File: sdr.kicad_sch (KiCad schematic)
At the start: 9 parts, among them U1 IS42S86400F-7TL

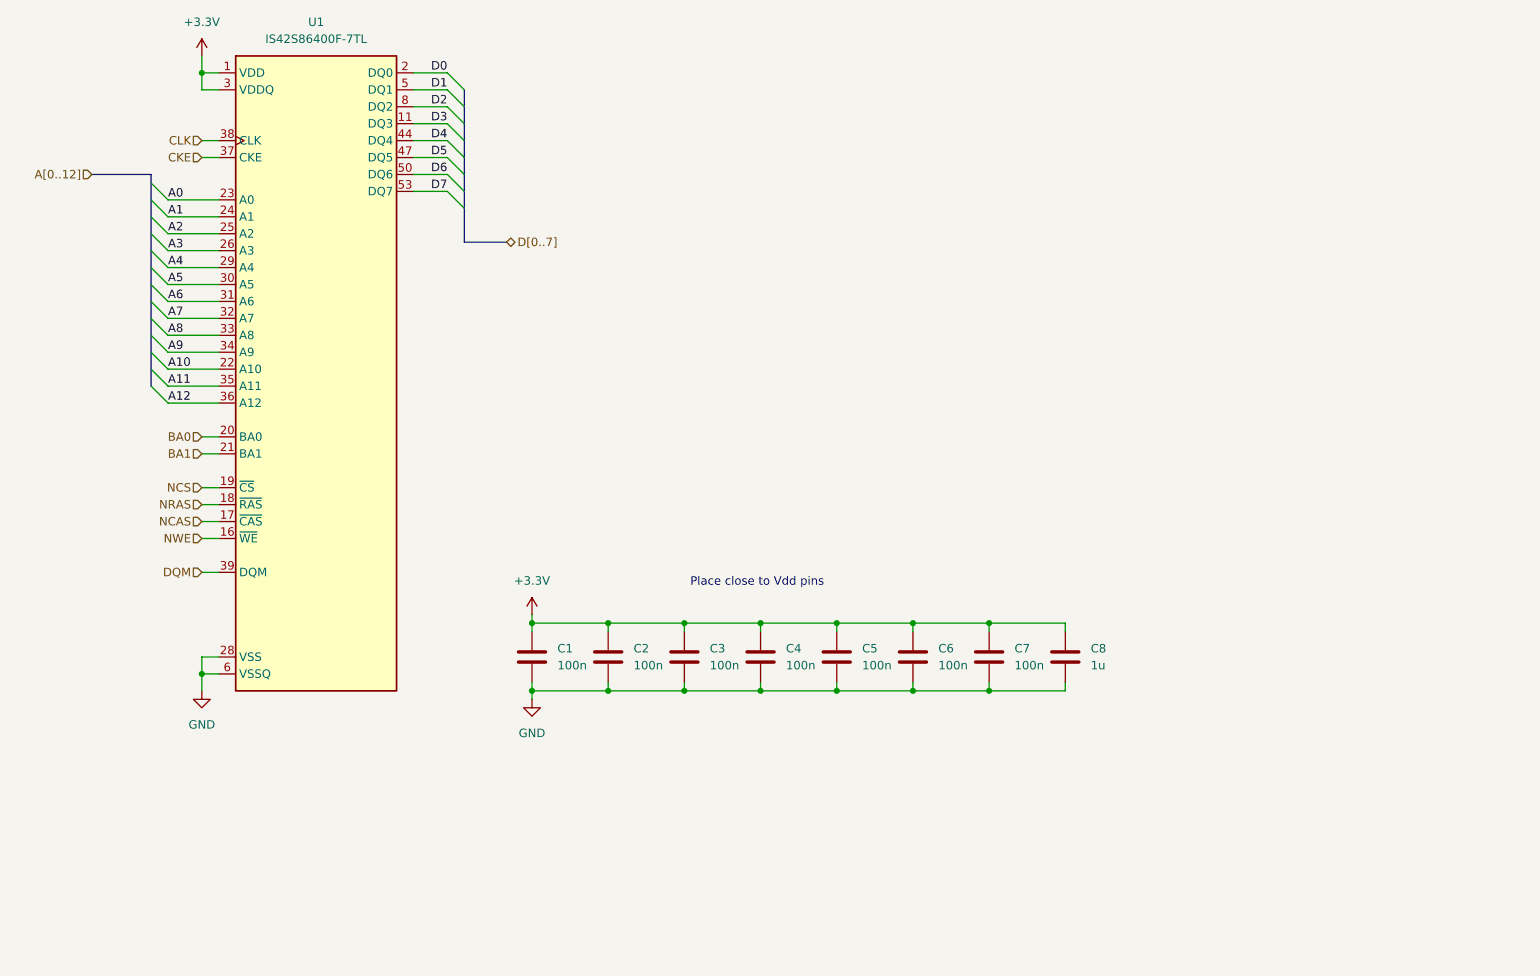
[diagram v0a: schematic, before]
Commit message: [#100650] Add rev number
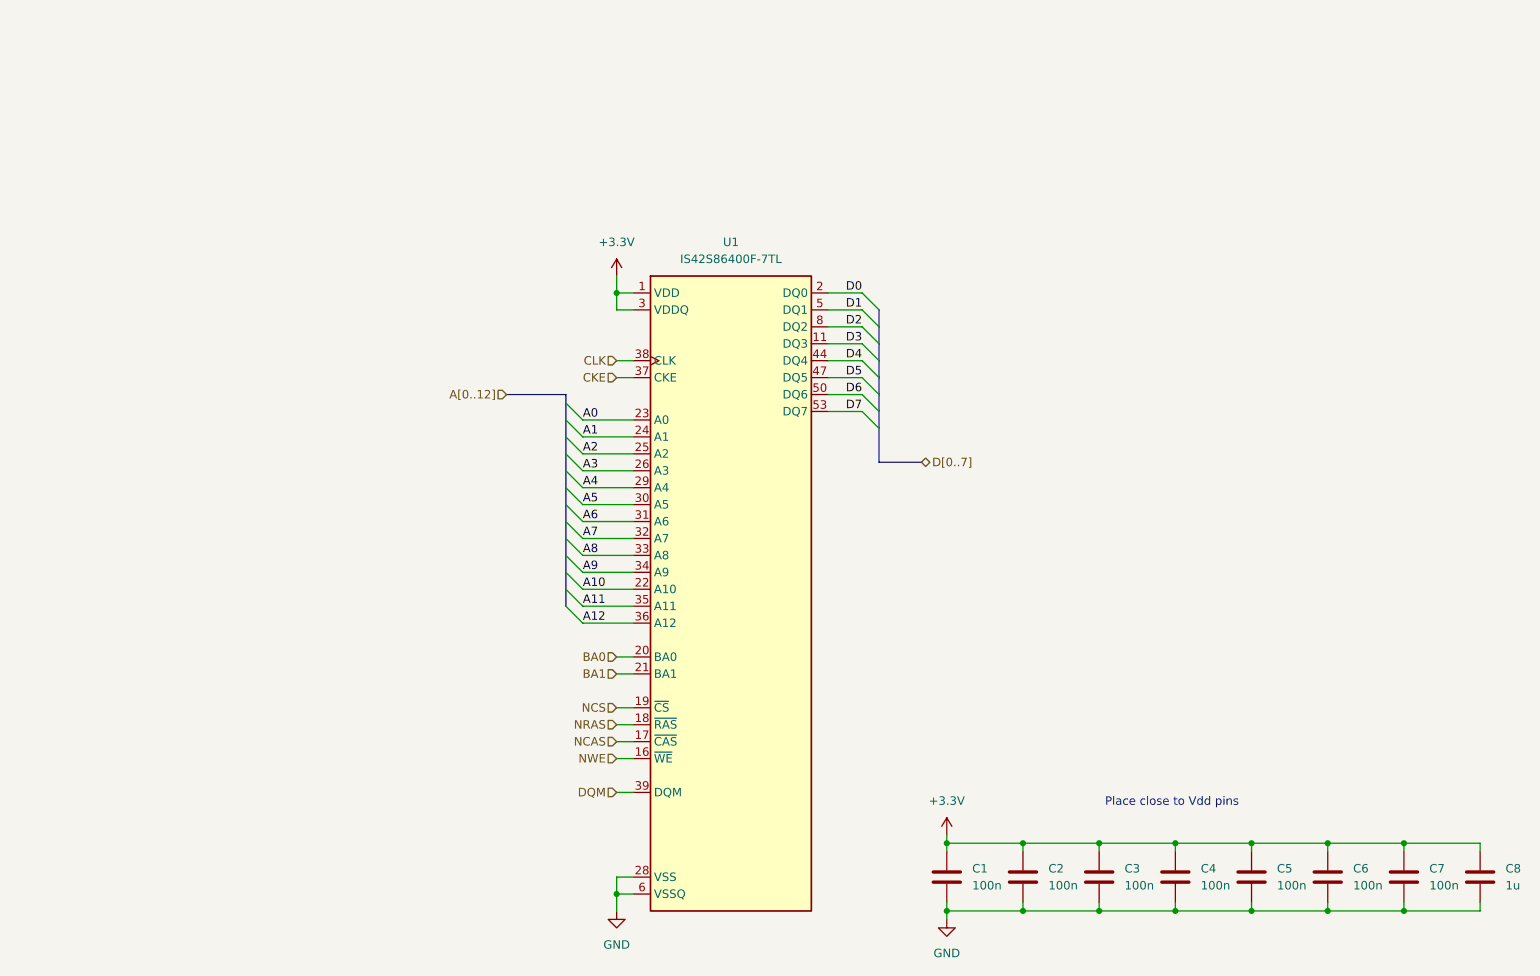
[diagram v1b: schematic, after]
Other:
- moved on the sheet: C1, C2, C3, C4, C5, C6, C7, C8, U1
